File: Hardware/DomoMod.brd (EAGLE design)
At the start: 80 x 30 mm, 46 parts, among them Q1 BSS138, Q2 BSS138, T1 MMBT2222A, U1 BD9251FV, U2 CCS811, U3 BME280, U4 PIR

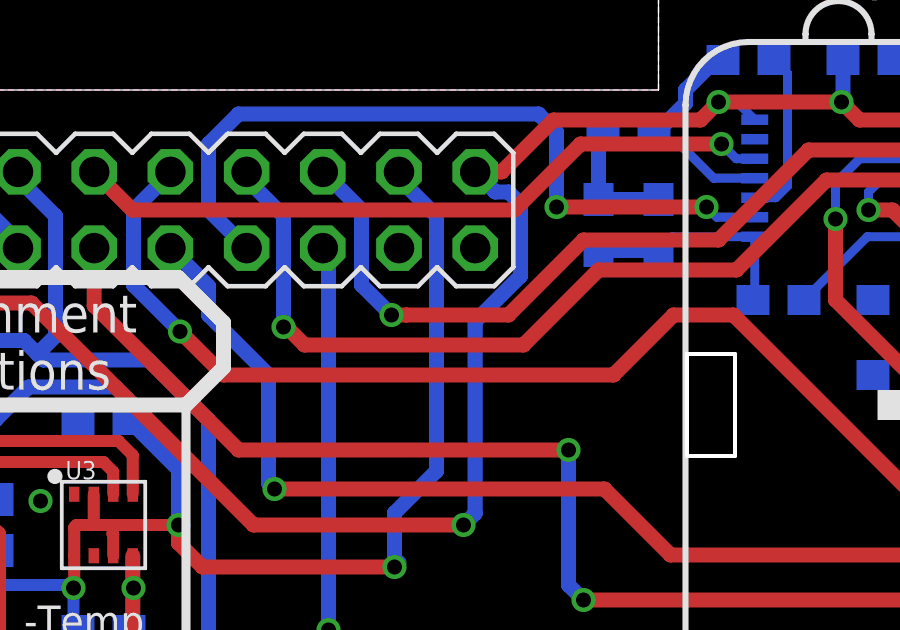
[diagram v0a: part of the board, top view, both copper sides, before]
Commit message: Updated design files
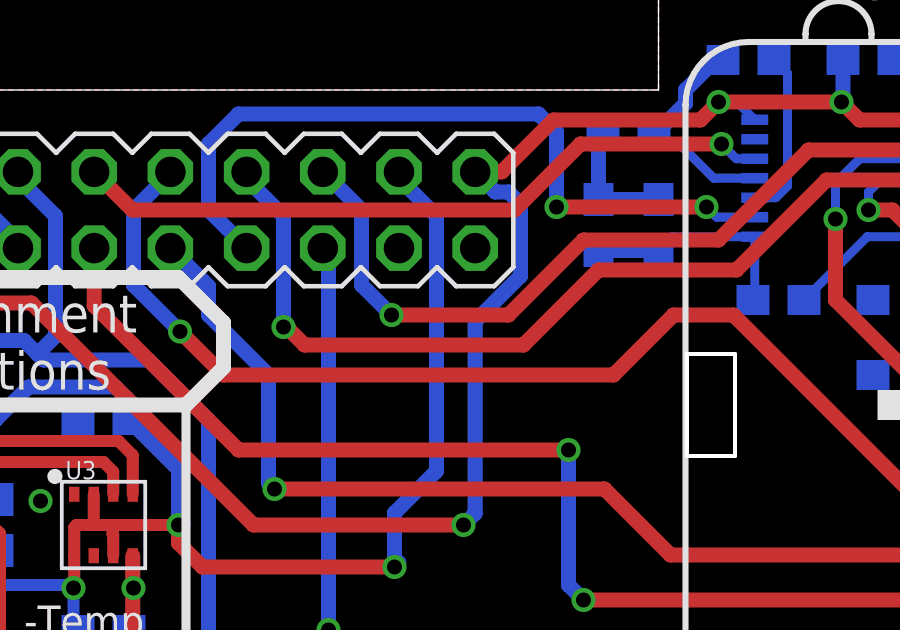
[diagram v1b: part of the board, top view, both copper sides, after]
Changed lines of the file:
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@@
 <signal name="D5">
 <wire x1="37.5" y1="19.5" x2="35" y2="17" width="0.5" layer="1"/>
-<wire x1="35" y1="17" x2="31.6" y2="17" width="0.5" layer="1"/>
+<wire x1="35" y1="17" x2="31.1" y2="17" width="0.5" layer="1"/>
 <wire x1="70.7" y1="19.5" x2="53.2" y2="19.5" width="0.5" layer="1"/>
 <wire x1="53.2" y1="19.5" x2="50.2" y2="22.5" width="0.5" layer="1"/>
@@
 <wire x1="30.1" y1="18" x2="31.1" y2="17" width="0.5" layer="16"/>
 <via x="31.1" y="17" extent="1-16" drill="0.5"/>
-<wire x1="31.1" y1="17" x2="31.6" y2="17" width="0.5" layer="1"/>
 </signal>
 <signal name="D6">
